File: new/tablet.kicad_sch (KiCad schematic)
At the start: 44 parts, among them J1 FSMC/TOUCH-SPI, J2 USB_B_Micro, J3 SD/CARD, J4 FLASH/FONT, J5 Conn_02x03_Odd_Even, J6 Conn_01x02, Q1 DMG2301L, SW1 SW_SPST, U1 STM32F429Z_E-G_Tx, U2 TPS63001, U3 MCP73811T-420I-OT, Y1 Crystal

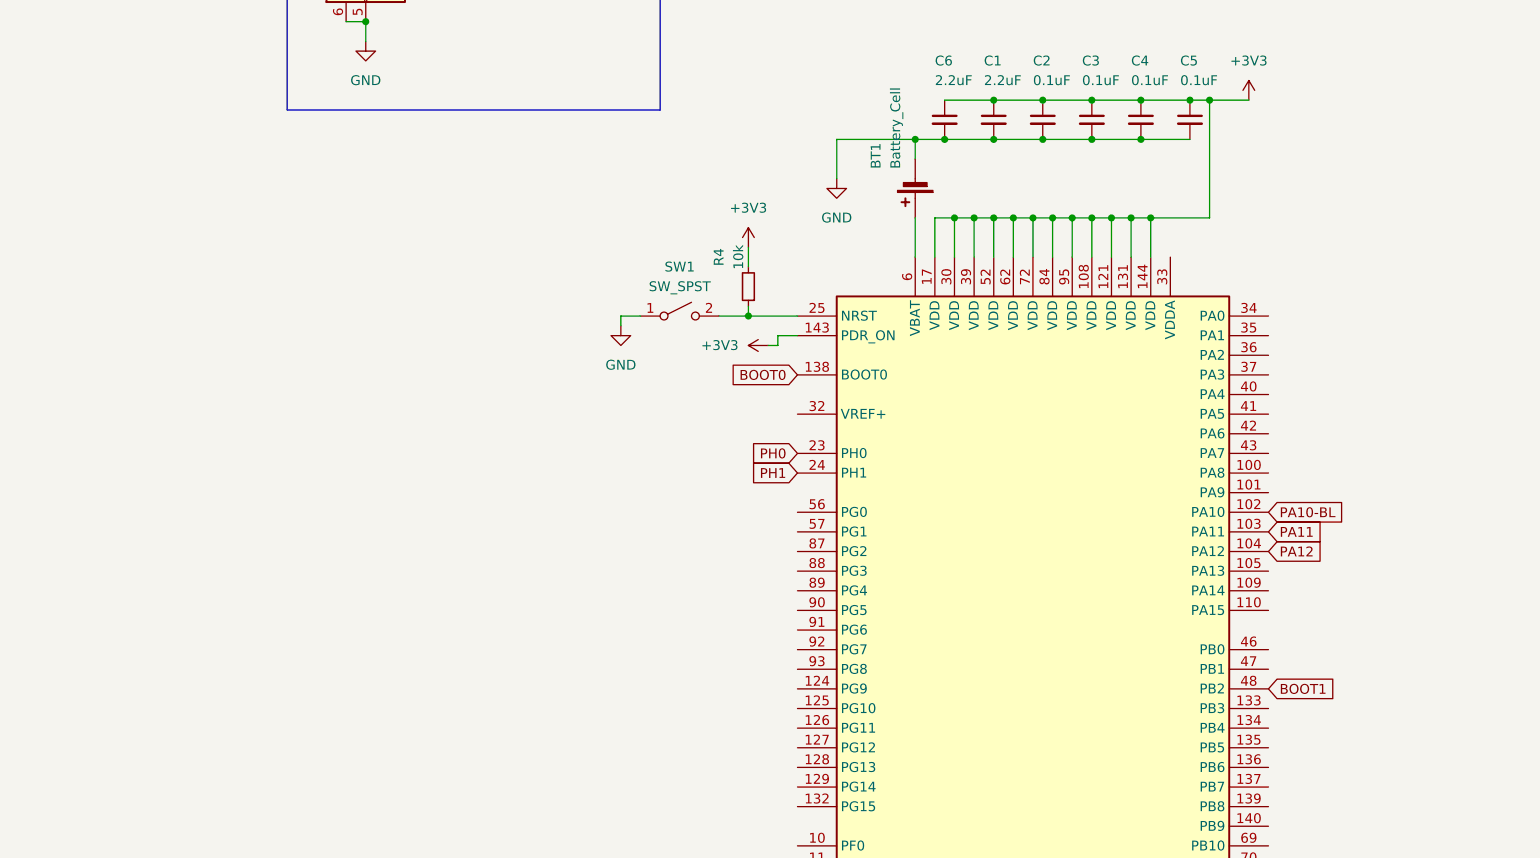
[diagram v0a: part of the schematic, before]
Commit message: wiring
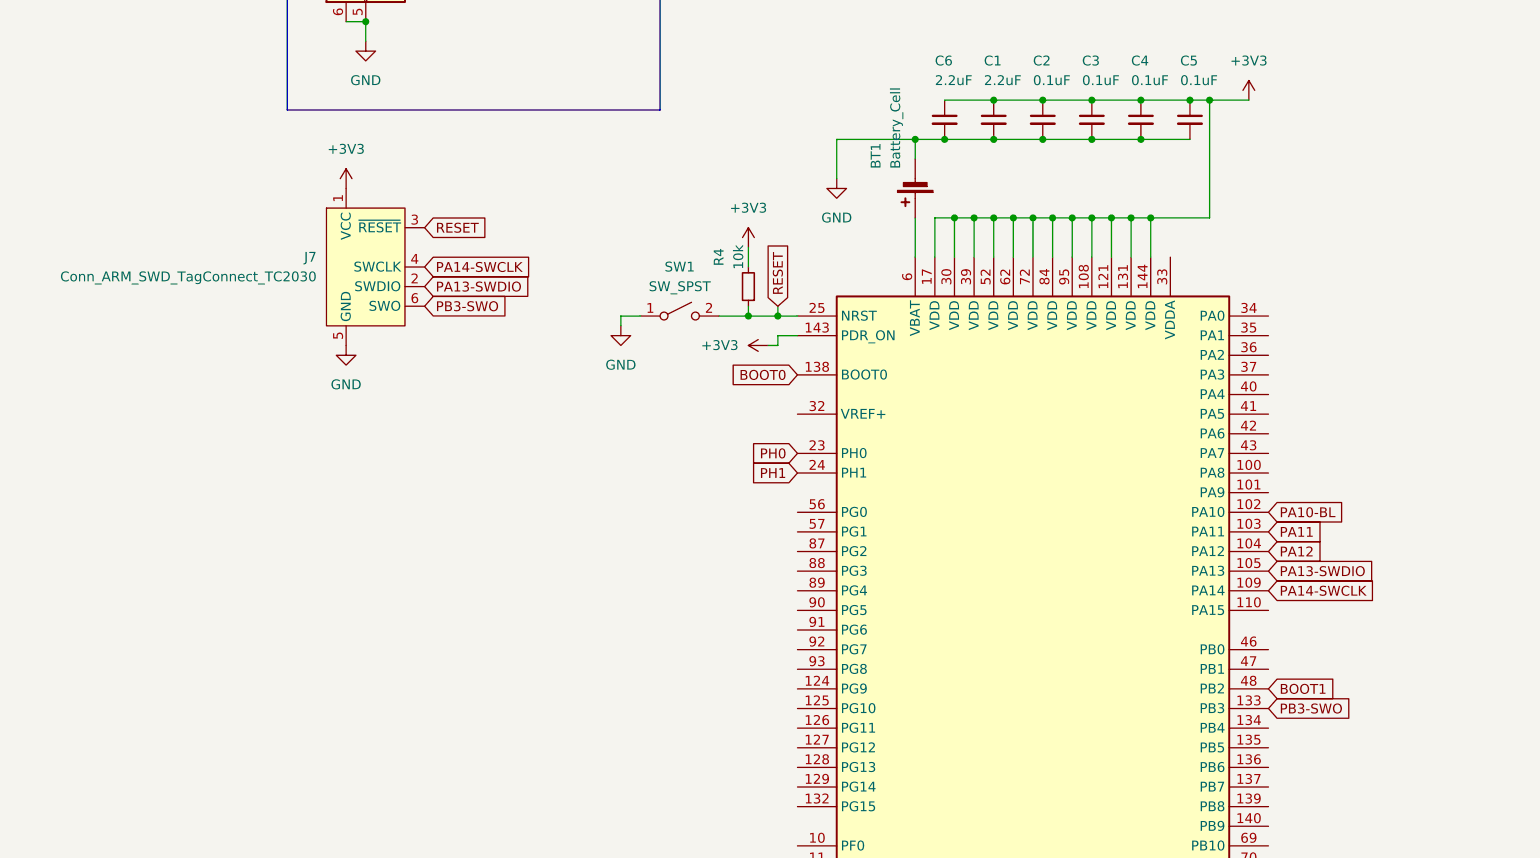
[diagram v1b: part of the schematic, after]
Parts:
- added J7: Conn_ARM_SWD_TagConnect_TC2030, Connector_PinHeader_2.54mm:PinHeader_1x06_P2.54mm_Vertical, symbol Connector:Conn_ARM_SWD_TagConnect_TC2030
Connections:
- net +3V3: now also J7.1 (VCC)
- net GND: now also J7.5 (GND)
- net RESET: now reaches R4.1, SW1.2 (B), U1.25 (NRST)
- net RESET: now also J7.3 (~{RESET})
- net PA13-SWDIO: now reaches U1.105 (PA13)
- net PA13-SWDIO: now also J7.2 (SWDIO)
- net PA14-SWCLK: now reaches U1.109 (PA14)
- net PA14-SWCLK: now also J7.4 (SWCLK)
- net PB3-SWO: now reaches U1.133 (PB3)
- net PB3-SWO: now also J7.6 (SWO)
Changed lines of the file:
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@@
   (junction (at 336.55 53.34) (diameter 0) (color 0 0 0 0)
   )
+  (junction (at 76.2 80.01) (diameter 0) (color 0 0 0 0)
+  )
   (junction (at 116.84 52.07) (diameter 0) (color 0 0 0 0)
   )
@@
     (stroke (width 0) (type default))
   )
+  (wire (pts (xy 76.2 80.01) (xy 78.74 80.01))
+    (stroke (width 0) (type default))
+  )
   (wire (pts (xy 347.98 73.66) (xy 347.98 83.82))
     (stroke (width 0) (type default))
@@
     (stroke (width 0) (type default))
   )
-  (wire (pts (xy 72.39 80.01) (xy 78.74 80.01))
+  (wire (pts (xy 72.39 80.01) (xy 76.2 80.01))
     (stroke (width 0) (type default))
   )
@@
   )
   (wire (pts (xy 341.63 72.39) (xy 341.63 63.5))
+    (stroke (width 0) (type default))
+  )
+  (wire (pts (xy 76.2 78.74) (xy 76.2 80.01))
     (stroke (width 0) (type default))
   )
@@
     )
   )
+  (global_label "PA13-SWDIO" (shape input) (at 139.7 113.03 0) (fields_autoplaced)
+    (effects (font (size 1.27 1.27)) (justify left))
+    (property "Intersheetrefs" "${INTERSHEET_REFS}" (at 154.9014 113.03 0)
+      (effects (font (size 1.27 1.27)) (justify left) hide)
+    )
+  )
   (global_label "PC10-DAT2" (shape input) (at 243.84 96.52 0) (fields_autoplaced)
     (effects (font (size 1.27 1.27)) (justify left))
@@
     )
   )
+  (global_label "PB3-SWO" (shape input) (at 30.48 78.74 0) (fields_autoplaced)
+    (effects (font (size 1.27 1.27)) (justify left))
+    (property "Intersheetrefs" "${INTERSHEET_REFS}" (at 42.7785 78.74 0)
+      (effects (font (size 1.27 1.27)) (justify left) hide)
+    )
+  )
   (global_label "BOOT1" (shape input) (at 139.7 128.27 0) (fields_autoplaced)
     (effects (font (size 1.27 1.27)) (justify left))
@@
     )
   )
+  (global_label "RESET" (shape input) (at 30.48 68.58 0) (fields_autoplaced)
+    (effects (font (size 1.27 1.27)) (justify left))
+    (property "Intersheetrefs" "${INTERSHEET_REFS}" (at 39.2103 68.58 0)
+      (effects (font (size 1.27 1.27)) (justify left) hide)
+    )
+  )
+  (global_label "PA14-SWCLK" (shape input) (at 139.7 115.57 0) (fields_autoplaced)
+    (effects (font (size 1.27 1.27)) (justify left))
+    (property "Intersheetrefs" "${INTERSHEET_REFS}" (at 155.2642 115.57 0)
+      (effects (font (size 1.27 1.27)) (justify left) hide)
+    )
+  )
   (global_label "PE8-D5" (shape input) (at 78.74 212.09 180) (fields_autoplaced)
     (effects (font (size 1.27 1.27)) (justify right))
@@
     )
   )
+  (global_label "PA14-SWCLK" (shape input) (at 30.48 73.66 0) (fields_autoplaced)
+    (effects (font (size 1.27 1.27)) (justify left))
+    (property "Intersheetrefs" "${INTERSHEET_REFS}" (at 46.0442 73.66 0)
+      (effects (font (size 1.27 1.27)) (justify left) hide)
+    )
+  )
   (global_label "PH1" (shape input) (at 191.77 125.73 90) (fields_autoplaced)
     (effects (font (size 1.27 1.27)) (justify left))
@@
     )
   )
+  (global_label "RESET" (shape input) (at 76.2 78.74 90) (fields_autoplaced)
+    (effects (font (size 1.27 1.27)) (justify left))
+    (property "Intersheetrefs" "${INTERSHEET_REFS}" (at 76.2 70.0097 90)
+      (effects (font (size 1.27 1.27)) (justify left) hide)
+    )
+  )
   (global_label "PD11-RS" (shape input) (at 139.7 237.49 0) (fields_autoplaced)
     (effects (font (size 1.27 1.27)) (justify left))
@@
     )
   )
+  (global_label "PB3-SWO" (shape input) (at 139.7 130.81 0) (fields_autoplaced)
+    (effects (font (size 1.27 1.27)) (justify left))
+    (property "Intersheetrefs" "${INTERSHEET_REFS}" (at 151.9985 130.81 0)
+      (effects (font (size 1.27 1.27)) (justify left) hide)
+    )
+  )
   (global_label "PB12-TP{slash}CS" (shape input) (at 139.7 153.67 0) (fields_autoplaced)
     (effects (font (size 1.27 1.27)) (justify left))
@@
     (property "Intersheetrefs" "${INTERSHEET_REFS}" (at 65.6554 224.79 0)
       (effects (font (size 1.27 1.27)) (justify right) hide)
+    )
+  )
+  (global_label "PA13-SWDIO" (shape input) (at 30.48 76.2 0) (fields_autoplaced)
+    (effects (font (size 1.27 1.27)) (justify left))
+    (property "Intersheetrefs" "${INTERSHEET_REFS}" (at 45.6814 76.2 0)
+      (effects (font (size 1.27 1.27)) (justify left) hide)
     )
   )
@@
     )
   )
+  (symbol (lib_id "power:GND") (at 20.32 83.82 0) (unit 1)
+    (in_bom yes) (on_board yes) (dnp no) (fields_autoplaced)
+    (property "Reference" "#PWR030" (at 20.32 90.17 0)
+      (effects (font (size 1.27 1.27)) hide)
+    )
+    (property "Value" "GND" (at 20.32 88.9 0)
+      (effects (font (size 1.27 1.27)))
+    )
+    (property "Footprint" "" (at 20.32 83.82 0)
+      (effects (font (size 1.27 1.27)) hide)
+    )
+    (property "Datasheet" "" (at 20.32 83.82 0)
+      (effects (font (size 1.27 1.27)) hide)
+    )
+    (pin "1")
+    (instances
+      (project "tablet"
+        (path "/868516f5-1ea3-47ae-b277-3f67998564bb"
+          (reference "#PWR030") (unit 1)
+        )
+      )
+    )
+  )
   (symbol (lib_id "power:+BATT") (at 363.22 110.49 0) (unit 1)
     (in_bom yes) (on_board yes) (dnp no) (fields_autoplaced)
@@
         (path "/868516f5-1ea3-47ae-b277-3f67998564bb"
           (reference "R7") (unit 1)
+        )
+      )
+    )
+  )
+  (symbol (lib_id "power:+3V3") (at 20.32 63.5 0) (unit 1)
+    (in_bom yes) (on_board yes) (dnp no) (fields_autoplaced)
+    (property "Reference" "#PWR029" (at 20.32 67.31 0)
+      (effects (font (size 1.27 1.27)) hide)
+    )
+    (property "Value" "+3V3" (at 20.32 58.42 0)
+      (effects (font (size 1.27 1.27)))
+    )
+    (property "Footprint" "" (at 20.32 63.5 0)
+      (effects (font (size 1.27 1.27)) hide)
+    )
+    (property "Datasheet" "" (at 20.32 63.5 0)
+      (effects (font (size 1.27 1.27)) hide)
+    )
+    (pin "1")
+    (instances
+      (project "tablet"
+        (path "/868516f5-1ea3-47ae-b277-3f67998564bb"
+          (reference "#PWR029") (unit 1)
         )
       )
@@
         )
       )
+    )
+  )
+  (symbol (lib_id "Connector:Conn_ARM_SWD_TagConnect_TC2030") (at 22.86 73.66 0) (unit 1)
+    (in_bom no) (on_board yes) (dnp no) (fields_autoplaced)
+    (property "Reference" "J7" (at 16.51 72.39 0)
+      (effects (font (size 1.27 1.27)) (justify right))
+    )
+    (property "Value" "Conn_ARM_SWD_TagConnect_TC2030" (at 16.51 74.93 0)
+      (effects (font (size 1.27 1.27)) (justify right))
+    )
+    (property "Footprint" "Connector_PinHeader_2.54mm:PinHeader_1x06_P2.54mm_Vertical" (at 22.86 91.44 0)
+      (effects (font (size 1.27 1.27)) hide)
+    )
+    (property "Datasheet" "https://www.tag-connect.com/wp-content/uploads/bsk-pdf-manager/TC2030-CTX_1.pdf" (at 22.86 88.9 0)
+      (effects (font (size 1.27 1.27)) hide)
+    )
+    (pin "1")
+    (pin "2")
+    (pin "3")
+    (pin "4")
+    (pin "5")
+    (pin "6")
+    (instances
+      (project "tablet"
+        (path "/868516f5-1ea3-47ae-b277-3f67998564bb"
+          (reference "J7") (unit 1)
+        )
+      )

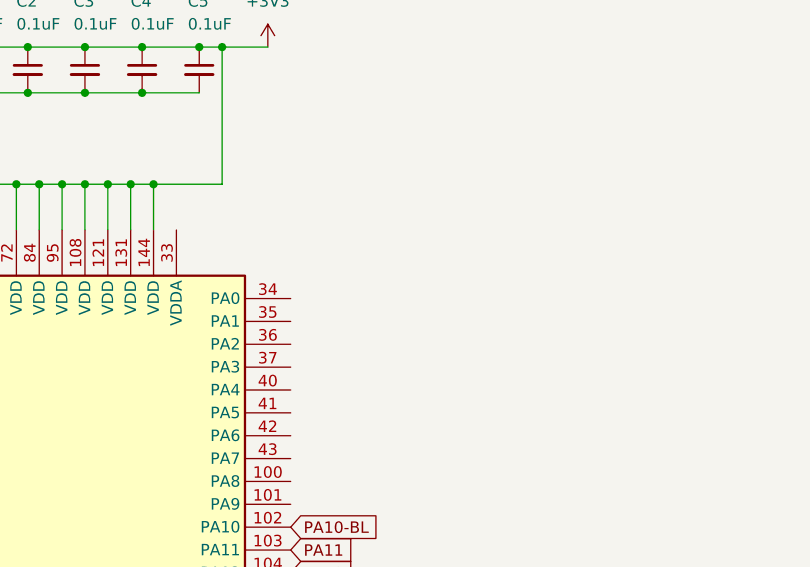
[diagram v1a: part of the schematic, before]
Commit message: add led
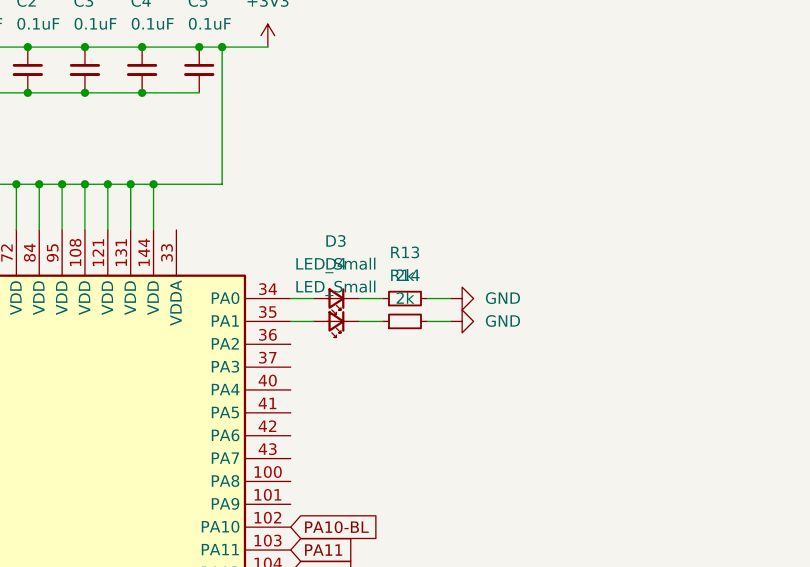
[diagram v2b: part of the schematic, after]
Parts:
- added D3, D4: LED_Small, Resistor_SMD:R_0603_1608Metric, symbol Device:LED_Small
- added R13, R14: 2k, Resistor_SMD:R_0603_1608Metric, symbol Device:R_Small
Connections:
- net GND: now also R13.2, R14.2
- net at U1.34 (PA0): now also D3.2 (A)
- net at U1.35 (PA1): now also D4.2 (A)
- new net: D4.1 (K), R14.1
- new net: D3.1 (K), R13.1
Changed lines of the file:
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@@
+    (stroke (width 0) (type default))
+  )
+  (wire (pts (xy 154.94 82.55) (xy 157.48 82.55))
     (stroke (width 0) (type default))
   )
@@
     (stroke (width 0) (type default))
   )
+  (wire (pts (xy 139.7 82.55) (xy 142.24 82.55))
+    (stroke (width 0) (type default))
+  )
   (wire (pts (xy 347.98 132.08) (xy 360.68 132.08))
     (stroke (width 0) (type default))
@@
     (stroke (width 0) (type default))
   )
+  (wire (pts (xy 147.32 80.01) (xy 149.86 80.01))
+    (stroke (width 0) (type default))
+  )
+  (wire (pts (xy 154.94 80.01) (xy 157.48 80.01))
+    (stroke (width 0) (type default))
+  )
+  (wire (pts (xy 142.24 80.01) (xy 139.7 80.01))
+    (stroke (width 0) (type default))
+  )
   (wire (pts (xy 116.84 30.48) (xy 119.38 30.48))
     (stroke (width 0) (type default))
@@
   )
   (wire (pts (xy 83.82 57.15) (xy 83.82 62.23))
+    (stroke (width 0) (type default))
+  )
+  (wire (pts (xy 147.32 82.55) (xy 149.86 82.55))
     (stroke (width 0) (type default))
   )
@@
         (path "/868516f5-1ea3-47ae-b277-3f67998564bb"
           (reference "C15") (unit 1)
+        )
+      )
+    )
+  )
+  (symbol (lib_id "power:GND") (at 157.48 82.55 90) (unit 1)
+    (in_bom yes) (on_board yes) (dnp no) (fields_autoplaced)
+    (property "Reference" "#PWR032" (at 163.83 82.55 0)
+      (effects (font (size 1.27 1.27)) hide)
+    )
+    (property "Value" "GND" (at 161.29 82.55 90)
+      (effects (font (size 1.27 1.27)) (justify right))
+    )
+    (property "Footprint" "" (at 157.48 82.55 0)
+      (effects (font (size 1.27 1.27)) hide)
+    )
+    (property "Datasheet" "" (at 157.48 82.55 0)
+      (effects (font (size 1.27 1.27)) hide)
+    )
+    (pin "1")
+    (instances
+      (project "tablet"
+        (path "/868516f5-1ea3-47ae-b277-3f67998564bb"
+          (reference "#PWR032") (unit 1)
         )
       )
@@
     )
   )
+  (symbol (lib_id "Device:LED_Small") (at 144.78 82.55 180) (unit 1)
+    (in_bom yes) (on_board yes) (dnp no) (fields_autoplaced)
+    (property "Reference" "D4" (at 144.7165 76.2 0)
+      (effects (font (size 1.27 1.27)))
+    )
+    (property "Value" "LED_Small" (at 144.7165 78.74 0)
+      (effects (font (size 1.27 1.27)))
+    )
+    (property "Footprint" "Resistor_SMD:R_0603_1608Metric" (at 144.78 82.55 90)
+      (effects (font (size 1.27 1.27)) hide)
+    )
+    (property "Datasheet" "~" (at 144.78 82.55 90)
+      (effects (font (size 1.27 1.27)) hide)
+    )
+    (pin "1")
+    (pin "2")
+    (instances
+      (project "tablet"
+        (path "/868516f5-1ea3-47ae-b277-3f67998564bb"
+          (reference "D4") (unit 1)
+        )
+      )
+    )
+  )
   (symbol (lib_id "power:GND") (at 203.2 125.73 180) (unit 1)
     (in_bom yes) (on_board yes) (dnp no) (fields_autoplaced)
@@
         (path "/868516f5-1ea3-47ae-b277-3f67998564bb"
           (reference "R6") (unit 1)
+        )
+      )
+    )
+  )
+  (symbol (lib_id "power:GND") (at 157.48 80.01 90) (unit 1)
+    (in_bom yes) (on_board yes) (dnp no) (fields_autoplaced)
+    (property "Reference" "#PWR031" (at 163.83 80.01 0)
+      (effects (font (size 1.27 1.27)) hide)
+    )
+    (property "Value" "GND" (at 161.29 80.01 90)
+      (effects (font (size 1.27 1.27)) (justify right))
+    )
+    (property "Footprint" "" (at 157.48 80.01 0)
+      (effects (font (size 1.27 1.27)) hide)
+    )
+    (property "Datasheet" "" (at 157.48 80.01 0)
+      (effects (font (size 1.27 1.27)) hide)
+    )
+    (pin "1")
+    (instances
+      (project "tablet"
+        (path "/868516f5-1ea3-47ae-b277-3f67998564bb"
+          (reference "#PWR031") (unit 1)
         )
       )
@@
     )
   )
+  (symbol (lib_id "Device:R_Small") (at 152.4 80.01 90) (unit 1)
+    (in_bom yes) (on_board yes) (dnp no) (fields_autoplaced)
+    (property "Reference" "R13" (at 152.4 74.93 90)
+      (effects (font (size 1.27 1.27)))
+    )
+    (property "Value" "2k" (at 152.4 77.47 90)
+      (effects (font (size 1.27 1.27)))
+    )
+    (property "Footprint" "Resistor_SMD:R_0603_1608Metric" (at 152.4 80.01 0)
+      (effects (font (size 1.27 1.27)) hide)
+    )
+    (property "Datasheet" "~" (at 152.4 80.01 0)
+      (effects (font (size 1.27 1.27)) hide)
+    )
+    (pin "1")
+    (pin "2")
+    (instances
+      (project "tablet"
+        (path "/868516f5-1ea3-47ae-b277-3f67998564bb"
+          (reference "R13") (unit 1)
+        )
+      )
+      (project "drone"
+        (path "/8d172cff-266e-4e68-aa3f-17546d01ba91"
+          (reference "R11") (unit 1)
+        )
+      )
+    )
+  )
   (symbol (lib_id "Diode:BAT48JFILM") (at 327.66 43.18 180) (unit 1)
     (in_bom yes) (on_board yes) (dnp no) (fields_autoplaced)
@@
         (path "/868516f5-1ea3-47ae-b277-3f67998564bb"
           (reference "D1") (unit 1)
+        )
+      )
+    )
+  )
+  (symbol (lib_id "Device:LED_Small") (at 144.78 80.01 180) (unit 1)
+    (in_bom yes) (on_board yes) (dnp no) (fields_autoplaced)
+    (property "Reference" "D3" (at 144.7165 73.66 0)
+      (effects (font (size 1.27 1.27)))
+    )
+    (property "Value" "LED_Small" (at 144.7165 76.2 0)
+      (effects (font (size 1.27 1.27)))
+    )
+    (property "Footprint" "Resistor_SMD:R_0603_1608Metric" (at 144.78 80.01 90)
+      (effects (font (size 1.27 1.27)) hide)
+    )
+    (property "Datasheet" "~" (at 144.78 80.01 90)
+      (effects (font (size 1.27 1.27)) hide)
+    )
+    (pin "1")
+    (pin "2")
+    (instances
+      (project "tablet"
+        (path "/868516f5-1ea3-47ae-b277-3f67998564bb"
+          (reference "D3") (unit 1)
         )
       )
@@
         )
       )
+    )
+  )
+  (symbol (lib_id "Device:R_Small") (at 152.4 82.55 90) (unit 1)
+    (in_bom yes) (on_board yes) (dnp no) (fields_autoplaced)
+    (property "Reference" "R14" (at 152.4 77.47 90)
+      (effects (font (size 1.27 1.27)))
+    )
+    (property "Value" "2k" (at 152.4 80.01 90)
+      (effects (font (size 1.27 1.27)))
+    )
+    (property "Footprint" "Resistor_SMD:R_0603_1608Metric" (at 152.4 82.55 0)
+      (effects (font (size 1.27 1.27)) hide)
+    )
+    (property "Datasheet" "~" (at 152.4 82.55 0)
+      (effects (font (size 1.27 1.27)) hide)
+    )
+    (pin "1")
+    (pin "2")
+    (instances
+      (project "tablet"
+        (path "/868516f5-1ea3-47ae-b277-3f67998564bb"
+          (reference "R14") (unit 1)
+        )
+      )
+      (project "drone"
+        (path "/8d172cff-266e-4e68-aa3f-17546d01ba91"
+          (reference "R11") (unit 1)
+        )
+      )
